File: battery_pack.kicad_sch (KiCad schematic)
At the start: 5 parts

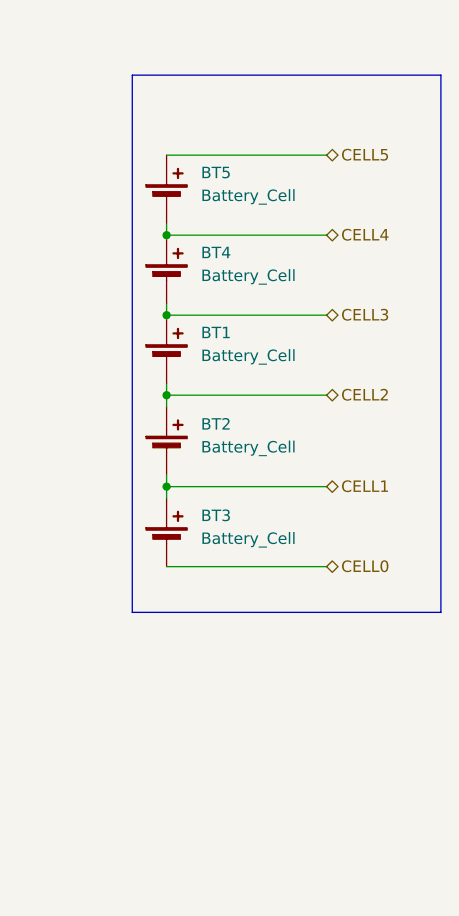
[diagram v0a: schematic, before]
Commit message: progress
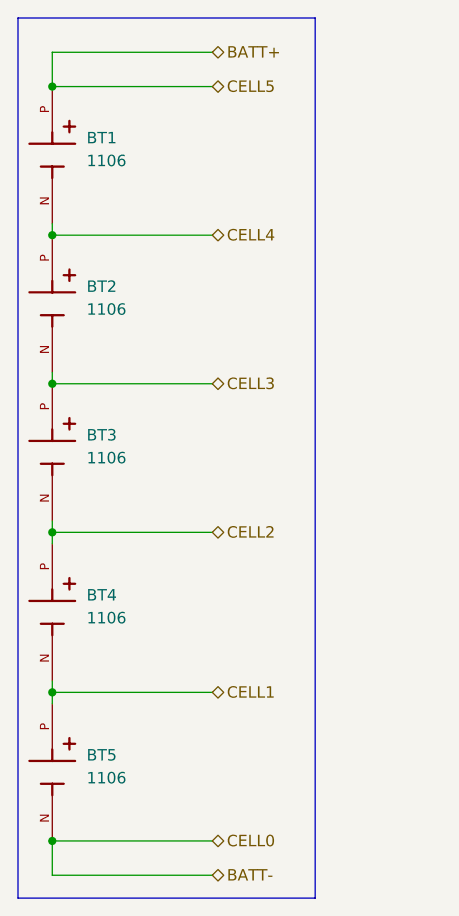
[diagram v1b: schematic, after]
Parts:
- removed BT1, BT2, BT3, BT4, BT5: Battery_Cell, symbol Device:Battery_Cell
- added BT1, BT2, BT3, BT4, BT5: 1106, 26650_cell_holder:BAT_1106, symbol 1106_26650_Cell_Holder:1106
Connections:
- net CELL1: now also BT4.N, BT5.P
- net CELL2: now also BT3.N, BT4.P
- net CELL3: now also BT2.N, BT3.P
- net CELL4: now also BT1.N, BT2.P
- new net BATT+: BT1.P
- new net BATT-: BT5.N
